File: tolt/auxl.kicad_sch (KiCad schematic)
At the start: 10 parts, among them J16 NRST, J17 NRST, U17 BMI160, U18 ESP32-C3-WROOM-02

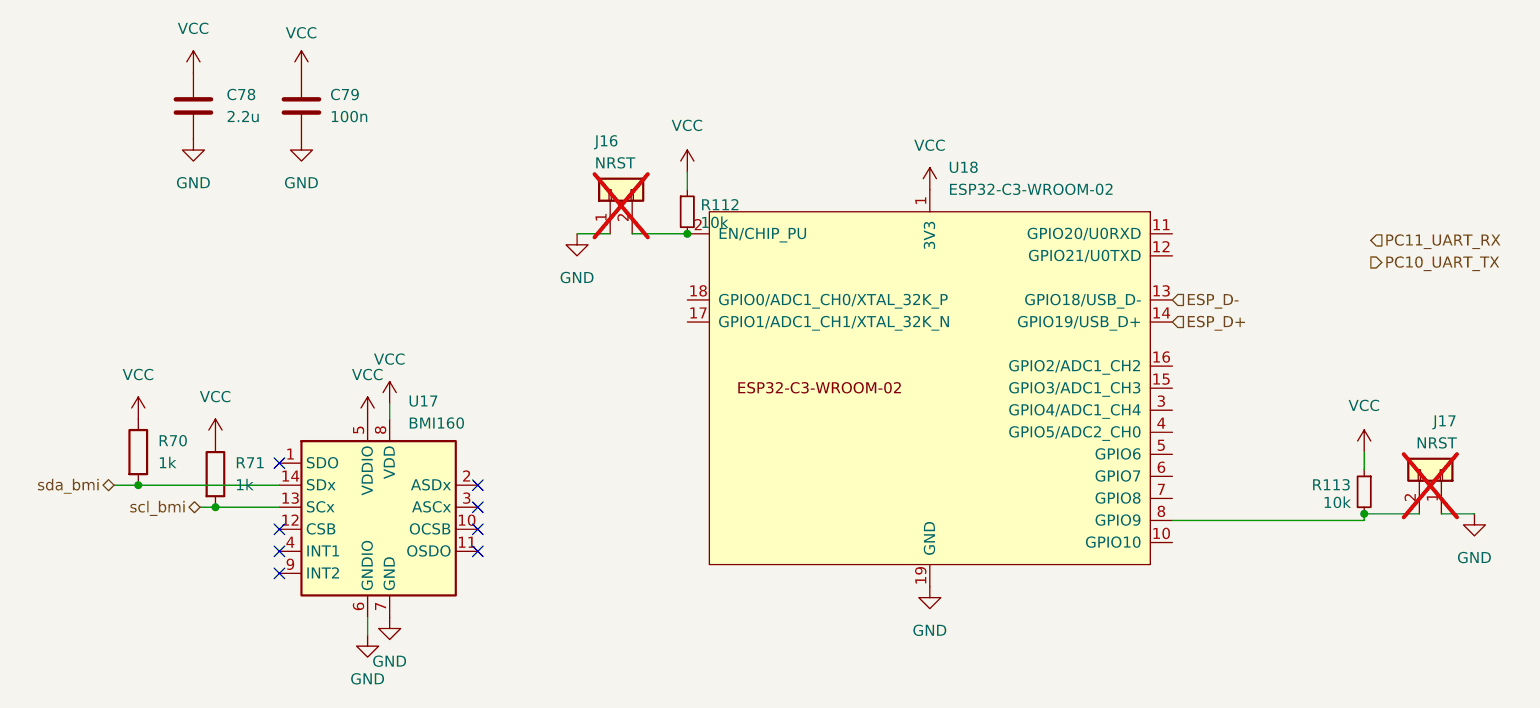
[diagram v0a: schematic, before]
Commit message: FINAL?
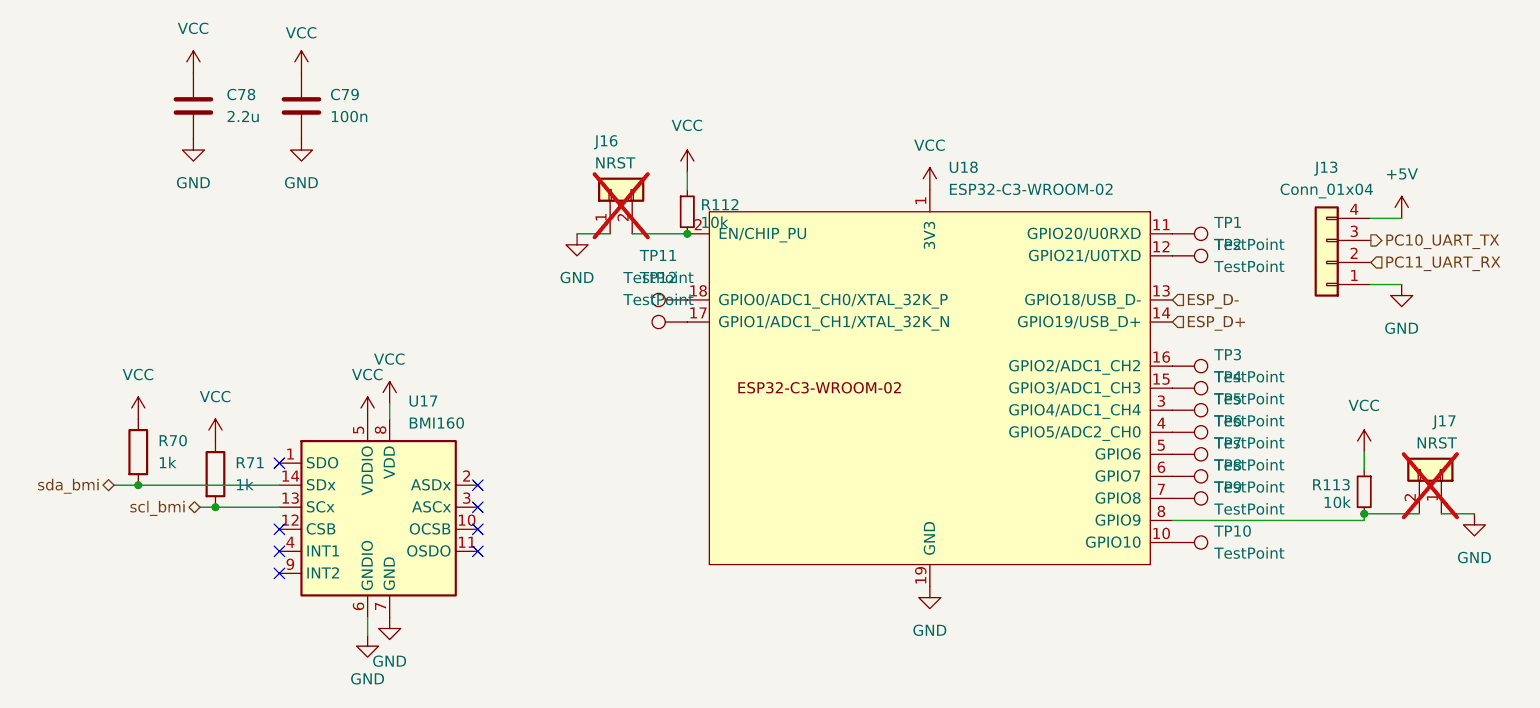
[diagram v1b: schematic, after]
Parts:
- added J13: Conn_01x04, Connector_JST:JST_PH_B4B-PH-K_1x04_P2.00mm_Vertical, symbol Connector_Generic:Conn_01x04
- added TP1, TP10, TP11, TP12, TP2, TP3, TP4, TP5, TP6, TP7, TP8, TP9: TestPoint, TestPoint:TestPoint_Pad_D1.0mm, symbol Connector:TestPoint
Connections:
- net GND: now also J13.1 (Pin_1)
- net PC10_UART_TX: now also J13.3 (Pin_3)
- net PC11_UART_RX: now also J13.2 (Pin_2)
- net at U18.10 (GPIO10): now also TP10.1
- net at U18.11 (GPIO20/U0RXD): now also TP1.1
- net at U18.12 (GPIO21/U0TXD): now also TP2.1
- net at U18.15 (GPIO3/ADC1_CH3): now also TP4.1
- net at U18.16 (GPIO2/ADC1_CH2): now also TP3.1
- net at U18.17 (GPIO1/ADC1_CH1/XTAL_32K_N): now also TP12.1
- net at U18.18 (GPIO0/ADC1_CH0/XTAL_32K_P): now also TP11.1
- net at U18.3 (GPIO4/ADC1_CH4): now also TP5.1
- net at U18.4 (GPIO5/ADC2_CH0): now also TP6.1
- net at U18.5 (GPIO6): now also TP7.1
- net at U18.6 (GPIO7): now also TP8.1
- net at U18.7 (GPIO8): now also TP9.1
- new net +5V: J13.4 (Pin_4)
